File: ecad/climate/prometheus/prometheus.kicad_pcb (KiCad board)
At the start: 2 copper layers, 34 x 44 mm, 13 parts, among them J1 2.5mm I.D. 5.5mm O.D., J2 5566-02A, J3 5566-02A, J4 5566-02A, J5 5566-02A

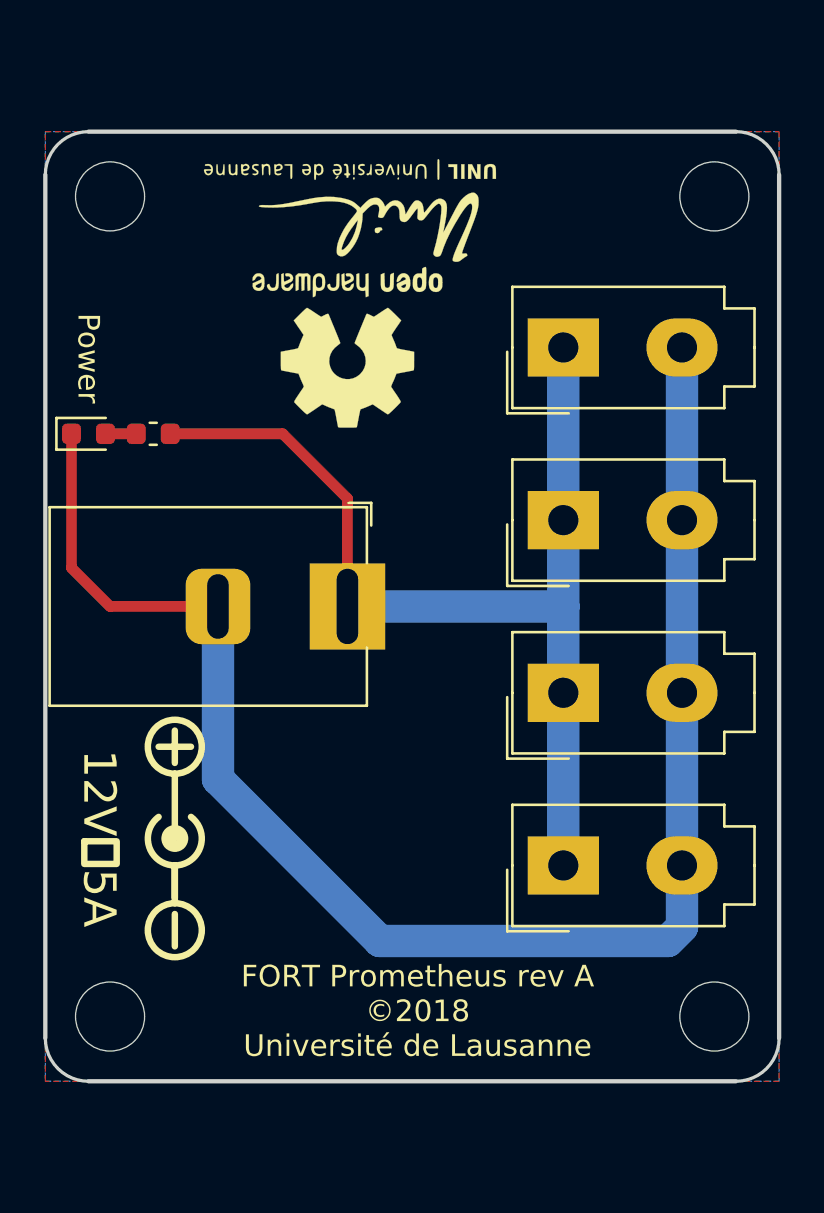
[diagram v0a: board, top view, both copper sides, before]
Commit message: Updates board for manufacturing
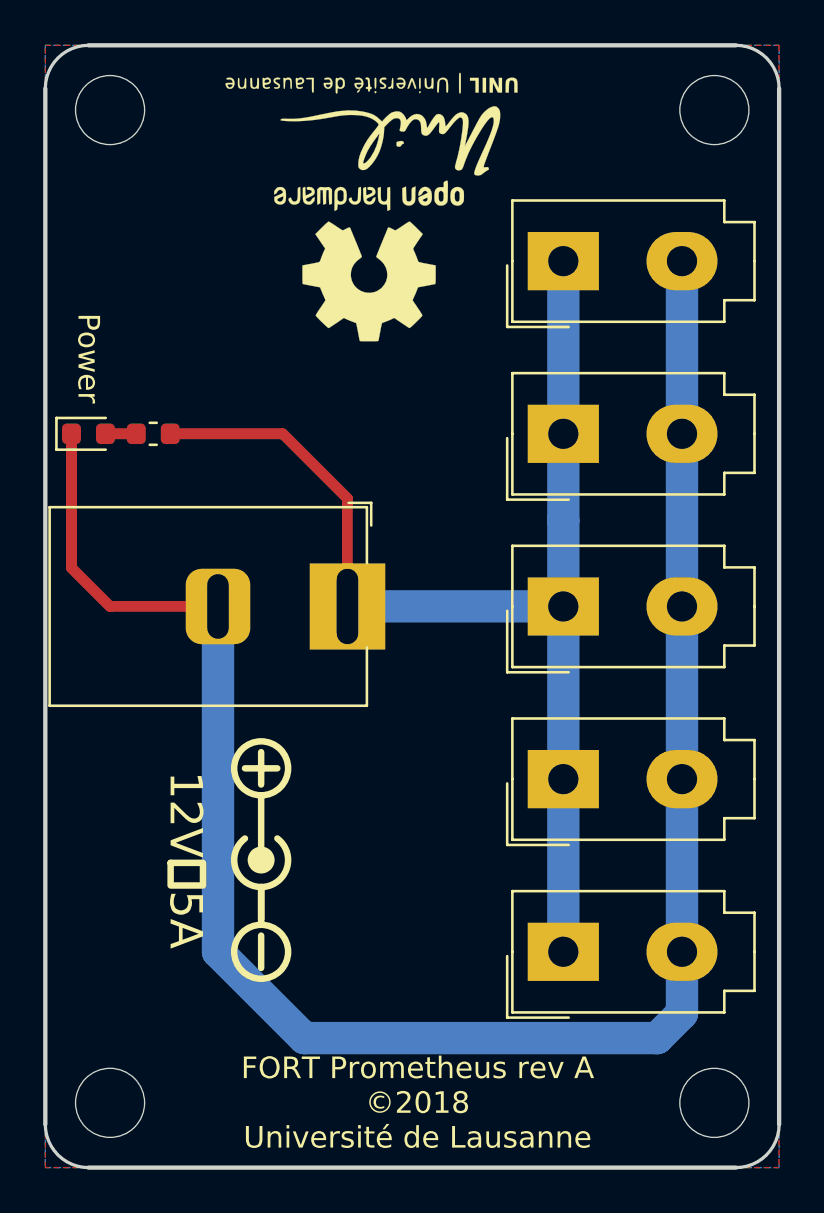
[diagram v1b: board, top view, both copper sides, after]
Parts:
- added J6: 5566-02A, Connector_Molex:Molex_Mini-Fit_Jr_5566-02A_2x01_P4.20mm_Vertical, F.Cu at (127.0, 116.0)
- moved G*** 4.12 mm to (118.0, 77.5)
- moved REF** 4.12 mm to (118.0, 84.0)
- moved J2 4.00 mm to (127.0, 84.0)
- moved J3 4.00 mm to (127.0, 92.0)
- moved J4 4.00 mm to (127.0, 100.0)
- moved J5 4.00 mm to (127.0, 108.0)
- moved MH1 4.00 mm to (106.0, 77.0)
- moved MH2 4.00 mm to (106.0, 123.0)
- moved MH3 4.00 mm to (134.0, 77.0)
- moved MH4 4.00 mm to (134.0, 123.0)
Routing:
- net GND: track 73.5 -> 88.2 mm
- net +12V: track 48.5 -> 56.5 mm
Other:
- board size 34 x 44 mm -> 34 x 52 mm
